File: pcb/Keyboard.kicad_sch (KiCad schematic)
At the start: 63 parts

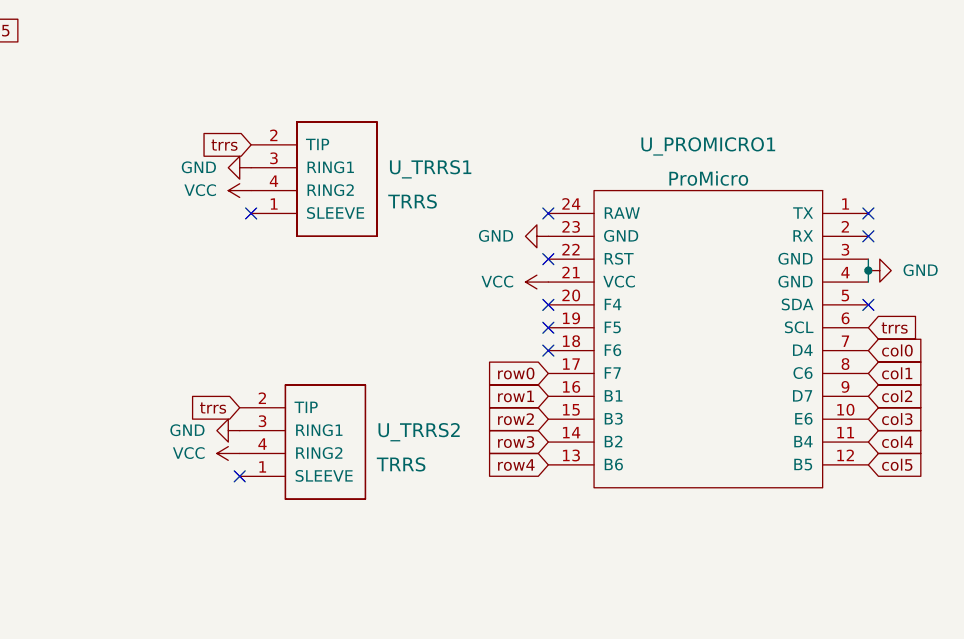
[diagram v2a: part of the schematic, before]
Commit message: wip
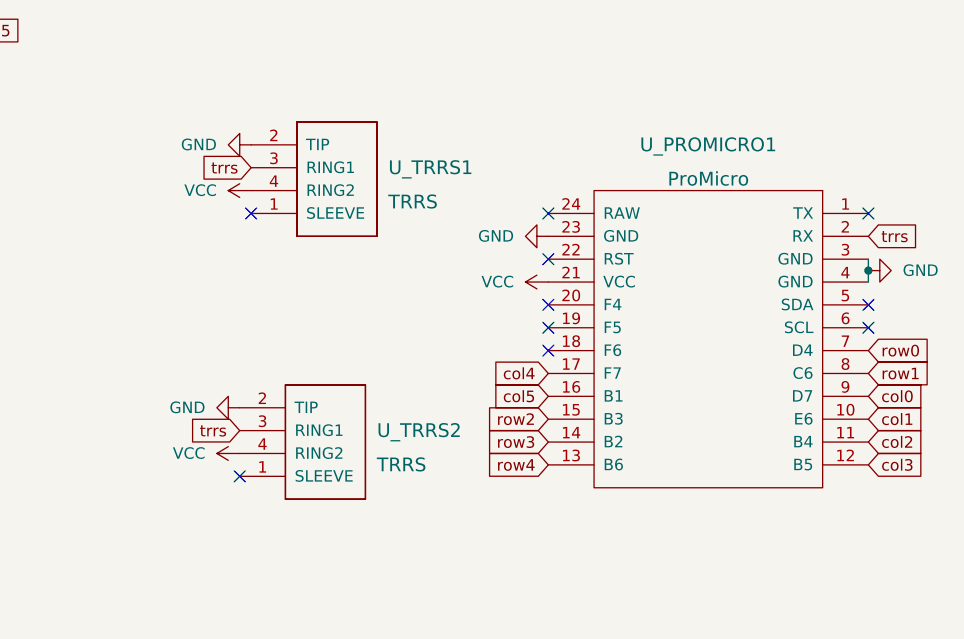
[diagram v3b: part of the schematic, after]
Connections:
- net GND: now also U_TRRS1.2 (TIP), U_TRRS2.2 (TIP); no longer U_TRRS1.3 (RING1), U_TRRS2.3 (RING1)
- net col0: now also U_PROMICRO1.9 (D7); no longer U_PROMICRO1.7 (D4)
- net col1: now also U_PROMICRO1.10 (E6); no longer U_PROMICRO1.8 (C6)
- net col2: now also U_PROMICRO1.11 (B4); no longer U_PROMICRO1.9 (D7)
- net col3: now also U_PROMICRO1.12 (B5); no longer U_PROMICRO1.10 (E6)
- net col4: now also U_PROMICRO1.17 (F7); no longer U_PROMICRO1.11 (B4)
- net col5: now also U_PROMICRO1.16 (B1); no longer U_PROMICRO1.12 (B5)
- net row0: now also U_PROMICRO1.7 (D4); no longer U_PROMICRO1.17 (F7)
- net row1: now also U_PROMICRO1.8 (C6); no longer U_PROMICRO1.16 (B1)
- net trrs: now also U_PROMICRO1.2 (RX), U_TRRS1.3 (RING1), U_TRRS2.3 (RING1); no longer U_PROMICRO1.6 (SCL), U_TRRS1.2 (TIP), U_TRRS2.2 (TIP)
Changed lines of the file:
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@@
   (no_connect (at 227.33 43.18))
   (no_connect (at 262.89 53.34))
-  (no_connect (at 262.89 45.72))
   (no_connect (at 262.89 43.18))
   (no_connect (at 227.33 58.42))
+  (no_connect (at 262.89 55.88))
   (no_connect (at 193.04 72.39))
   (no_connect (at 194.31 43.18))
@@
     (stroke (width 0) (type default) (color 0 0 0 0))
   )
-  (global_label "col5" (shape input) (at 262.89 71.12 0) (fields_autoplaced)
+  (global_label "col5" (shape input) (at 227.33 63.5 180) (fields_autoplaced)
+    (effects (font (size 1.27 1.27)) (justify right))
+    (property "Intersheet References" "${INTERSHEET_REFS}" (id 0) (at 220.8045 63.4206 0)
+      (effects (font (size 1.27 1.27)) (justify right) hide)
+    )
+  )
+  (global_label "col3" (shape input) (at 262.89 71.12 0) (fields_autoplaced)
     (effects (font (size 1.27 1.27)) (justify left))
     (property "Intersheet References" "${INTERSHEET_REFS}" (id 0) (at 269.4155 71.0406 0)
-      (effects (font (size 1.27 1.27)) (justify left) hide)
-    )
-  )
-  (global_label "col3" (shape input) (at 262.89 66.04 0) (fields_autoplaced)
-    (effects (font (size 1.27 1.27)) (justify left))
-    (property "Intersheet References" "${INTERSHEET_REFS}" (id 0) (at 269.4155 65.9606 0)
       (effects (font (size 1.27 1.27)) (justify left) hide)
     )
@@
     )
   )
-  (global_label "trrs" (shape input) (at 194.31 35.56 180) (fields_autoplaced)
+  (global_label "trrs" (shape input) (at 194.31 38.1 180) (fields_autoplaced)
     (effects (font (size 1.27 1.27)) (justify right))
-    (property "Intersheet References" "${INTERSHEET_REFS}" (id 0) (at 188.5707 35.4806 0)
+    (property "Intersheet References" "${INTERSHEET_REFS}" (id 0) (at 188.5707 38.0206 0)
       (effects (font (size 1.27 1.27)) (justify right) hide)
     )
@@
     )
   )
-  (global_label "trrs" (shape input) (at 262.89 55.88 0) (fields_autoplaced)
+  (global_label "trrs" (shape input) (at 262.89 45.72 0) (fields_autoplaced)
     (effects (font (size 1.27 1.27)) (justify left))
-    (property "Intersheet References" "${INTERSHEET_REFS}" (id 0) (at 268.6293 55.8006 0)
+    (property "Intersheet References" "${INTERSHEET_REFS}" (id 0) (at 268.6293 45.6406 0)
       (effects (font (size 1.27 1.27)) (justify left) hide)
     )
@@
     )
   )
-  (global_label "col2" (shape input) (at 262.89 63.5 0) (fields_autoplaced)
+  (global_label "col2" (shape input) (at 262.89 68.58 0) (fields_autoplaced)
     (effects (font (size 1.27 1.27)) (justify left))
-    (property "Intersheet References" "${INTERSHEET_REFS}" (id 0) (at 269.4155 63.4206 0)
+    (property "Intersheet References" "${INTERSHEET_REFS}" (id 0) (at 269.4155 68.5006 0)
       (effects (font (size 1.27 1.27)) (justify left) hide)
     )
@@
     )
   )
-  (global_label "col4" (shape input) (at 262.89 68.58 0) (fields_autoplaced)
-    (effects (font (size 1.27 1.27)) (justify left))
-    (property "Intersheet References" "${INTERSHEET_REFS}" (id 0) (at 269.4155 68.5006 0)
-      (effects (font (size 1.27 1.27)) (justify left) hide)
+  (global_label "col4" (shape input) (at 227.33 60.96 180) (fields_autoplaced)
+    (effects (font (size 1.27 1.27)) (justify right))
+    (property "Intersheet References" "${INTERSHEET_REFS}" (id 0) (at 220.8045 60.8806 0)
+      (effects (font (size 1.27 1.27)) (justify right) hide)
     )
   )
@@
     )
   )
-  (global_label "row0" (shape input) (at 227.33 60.96 180) (fields_autoplaced)
-    (effects (font (size 1.27 1.27)) (justify right))
-    (property "Intersheet References" "${INTERSHEET_REFS}" (id 0) (at 220.4417 60.8806 0)
-      (effects (font (size 1.27 1.27)) (justify right) hide)
+  (global_label "row0" (shape input) (at 262.89 58.42 0) (fields_autoplaced)
+    (effects (font (size 1.27 1.27)) (justify left))
+    (property "Intersheet References" "${INTERSHEET_REFS}" (id 0) (at 269.7783 58.3406 0)
+      (effects (font (size 1.27 1.27)) (justify left) hide)
     )
   )
@@
     )
   )
-  (global_label "col0" (shape input) (at 262.89 58.42 0) (fields_autoplaced)
+  (global_label "col0" (shape input) (at 262.89 63.5 0) (fields_autoplaced)
     (effects (font (size 1.27 1.27)) (justify left))
-    (property "Intersheet References" "${INTERSHEET_REFS}" (id 0) (at 269.4155 58.3406 0)
+    (property "Intersheet References" "${INTERSHEET_REFS}" (id 0) (at 269.4155 63.4206 0)
       (effects (font (size 1.27 1.27)) (justify left) hide)
     )
   )
-  (global_label "trrs" (shape input) (at 193.04 64.77 180) (fields_autoplaced)
+  (global_label "trrs" (shape input) (at 193.04 67.31 180) (fields_autoplaced)
     (effects (font (size 1.27 1.27)) (justify right))
-    (property "Intersheet References" "${INTERSHEET_REFS}" (id 0) (at 187.3007 64.6906 0)
+    (property "Intersheet References" "${INTERSHEET_REFS}" (id 0) (at 187.3007 67.2306 0)
       (effects (font (size 1.27 1.27)) (justify right) hide)
     )
   )
-  (global_label "row1" (shape input) (at 227.33 63.5 180) (fields_autoplaced)
-    (effects (font (size 1.27 1.27)) (justify right))
-    (property "Intersheet References" "${INTERSHEET_REFS}" (id 0) (at 220.4417 63.4206 0)
-      (effects (font (size 1.27 1.27)) (justify right) hide)
+  (global_label "row1" (shape input) (at 262.89 60.96 0) (fields_autoplaced)
+    (effects (font (size 1.27 1.27)) (justify left))
+    (property "Intersheet References" "${INTERSHEET_REFS}" (id 0) (at 269.7783 60.8806 0)
+      (effects (font (size 1.27 1.27)) (justify left) hide)
     )
   )
@@
     )
   )
-  (global_label "col1" (shape input) (at 262.89 60.96 0) (fields_autoplaced)
+  (global_label "col1" (shape input) (at 262.89 66.04 0) (fields_autoplaced)
     (effects (font (size 1.27 1.27)) (justify left))
-    (property "Intersheet References" "${INTERSHEET_REFS}" (id 0) (at 269.4155 60.8806 0)
+    (property "Intersheet References" "${INTERSHEET_REFS}" (id 0) (at 269.4155 65.9606 0)
       (effects (font (size 1.27 1.27)) (justify left) hide)
     )
@@
     (pin "1")
   )
-  (symbol (lib_id "power:GND") (at 193.04 67.31 270) (unit 1)
-    (in_bom yes) (on_board yes) (fields_autoplaced)
-    (property "Reference" "#PWR0102" (id 0) (at 186.69 67.31 0)
-      (effects (font (size 1.27 1.27)) hide)
-    )
-    (property "Value" "GND" (id 1) (at 189.23 67.3099 90)
-      (effects (font (size 1.27 1.27)) (justify right))
-    )
-    (property "Footprint" "" (id 2) (at 193.04 67.31 0)
-      (effects (font (size 1.27 1.27)) hide)
-    )
-    (property "Datasheet" "" (id 3) (at 193.04 67.31 0)
+  (symbol (lib_id "power:GND") (at 193.04 64.77 270) (unit 1)
+    (in_bom yes) (on_board yes)
+    (property "Reference" "#PWR0102" (id 0) (at 186.69 64.77 0)
+      (effects (font (size 1.27 1.27)) hide)
+    )
+    (property "Value" "GND" (id 1) (at 189.23 64.7699 90)
+      (effects (font (size 1.27 1.27)) (justify right))
+    )
+    (property "Footprint" "" (id 2) (at 193.04 64.77 0)
+      (effects (font (size 1.27 1.27)) hide)
+    )
+    (property "Datasheet" "" (id 3) (at 193.04 64.77 0)
       (effects (font (size 1.27 1.27)) hide)
     )
@@
     (pin "2")
   )
-  (symbol (lib_id "power:GND") (at 194.31 38.1 270) (unit 1)
-    (in_bom yes) (on_board yes) (fields_autoplaced)
-    (property "Reference" "#PWR0104" (id 0) (at 187.96 38.1 0)
-      (effects (font (size 1.27 1.27)) hide)
-    )
-    (property "Value" "GND" (id 1) (at 190.5 38.0999 90)
-      (effects (font (size 1.27 1.27)) (justify right))
-    )
-    (property "Footprint" "" (id 2) (at 194.31 38.1 0)
-      (effects (font (size 1.27 1.27)) hide)
-    )
-    (property "Datasheet" "" (id 3) (at 194.31 38.1 0)
-      (effects (font (size 1.27 1.27)) hide)
-    )
+  (symbol (lib_id "power:GND") (at 194.31 35.56 270) (unit 1)
+    (in_bom yes) (on_board yes) (fields_autoplaced)
+    (property "Reference" "#PWR0104" (id 0) (at 187.96 35.56 0)
+      (effects (font (size 1.27 1.27)) hide)
+    )
+    (property "Value" "GND" (id 1) (at 190.5 35.5599 90)
+      (effects (font (size 1.27 1.27)) (justify right))
+    )
+    (property "Footprint" "" (id 2) (at 194.31 35.56 0)
+      (effects (font (size 1.27 1.27)) hide)
+    )
+    (property "Datasheet" "" (id 3) (at 194.31 35.56 0)
+      (effects (font (size 1.27 1.27)) hide)
+    )

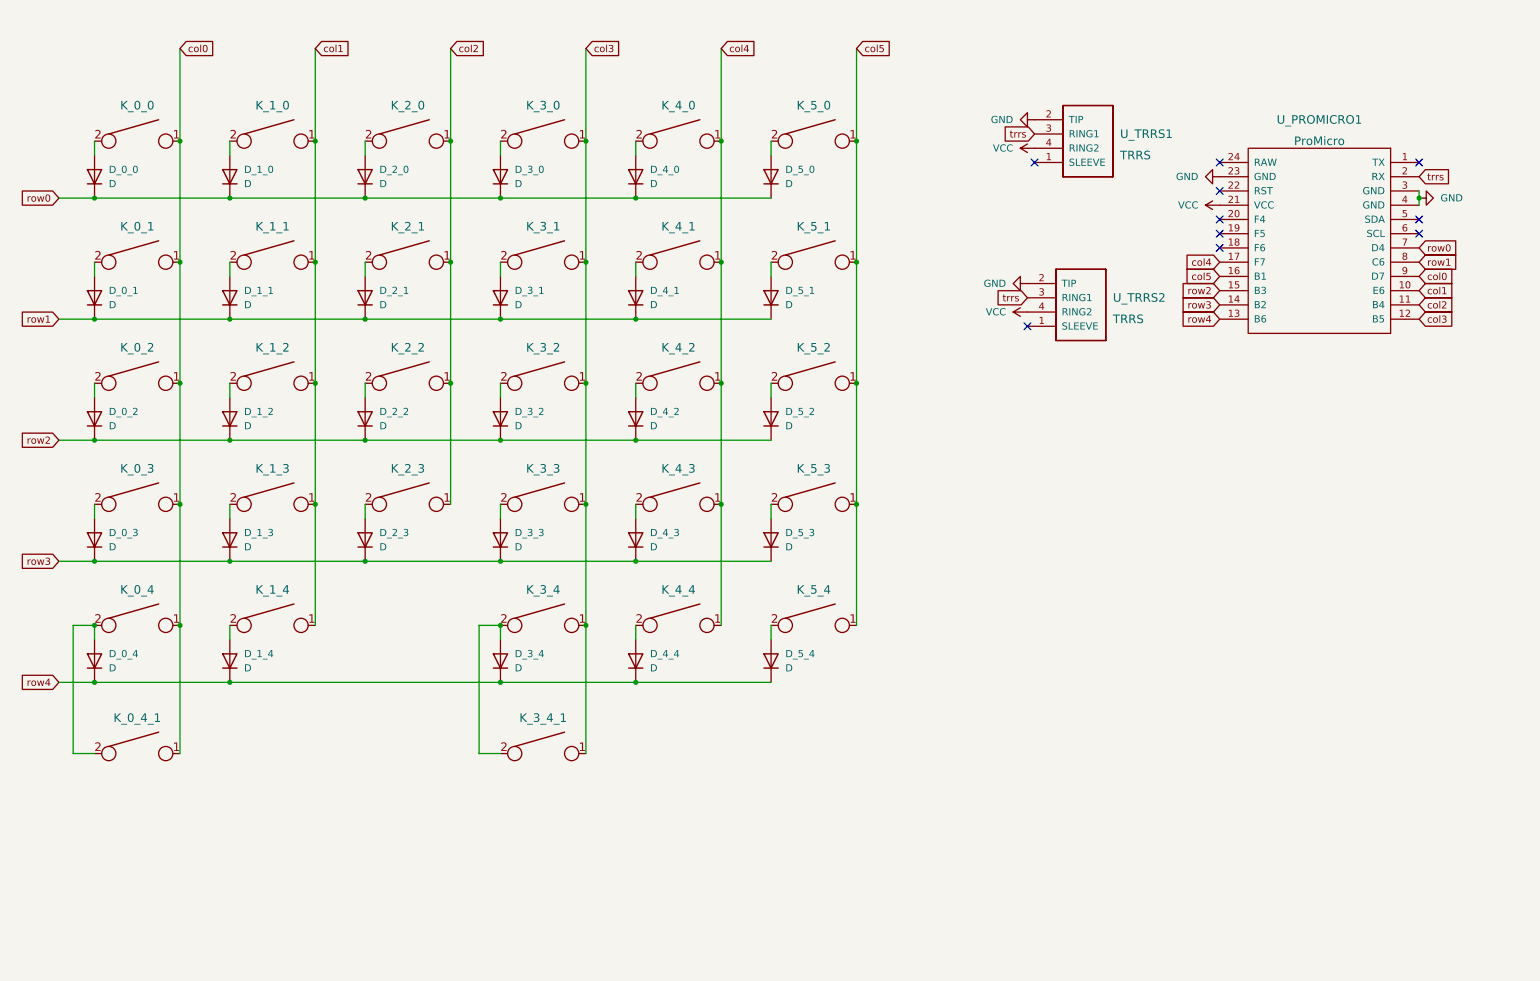
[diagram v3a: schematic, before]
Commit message: wip
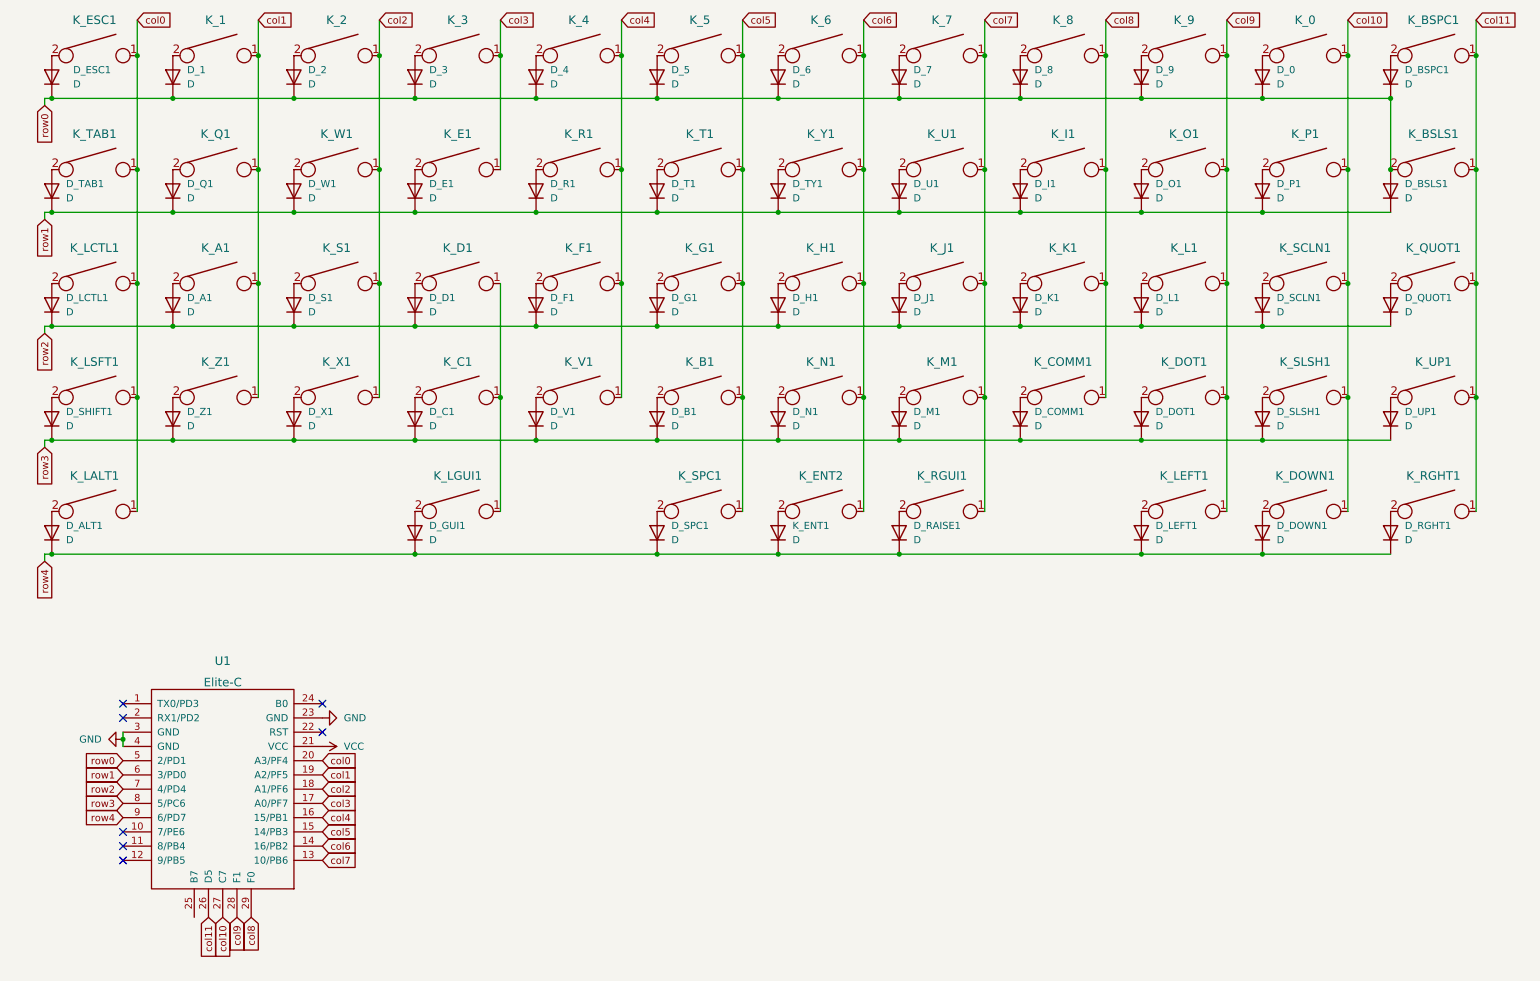
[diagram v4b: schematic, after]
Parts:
- removed D_0_4, D_1_4, D_3_4, D_4_4, D_5_4: D, keyboard_parts:D_SOD123, symbol Device:D
- removed K_0_4, K_0_4_1, K_1_4, K_3_4, K_3_4_1, K_4_4, K_5_4: KEYSW, Switch_Keyboard_Hotswap_Kailh:SW_Hotswap_Kailh_Choc_V1_1.00u, symbol keyboard_parts:KEYSW
- removed U_PROMICRO1: ProMicro, promicro:ProMicro, symbol promicro:ProMicro
- removed U_TRRS1, U_TRRS2: TRRS, Keebio-Parts:TRRS-PJ-320A, symbol keebio:TRRS
- added D_0, D_6, D_7, D_8, D_9, D_ALT1, D_BSLS1, D_BSPC1, D_COMM1, D_DOT1, D_DOWN1, D_GUI1, D_H1, D_I1, D_J1, D_K1, D_L1, D_LEFT1, D_M1, D_N1, D_O1, D_P1, D_QUOT1, D_RAISE1, D_RGHT1, D_SCLN1, D_SLSH1, D_SPC1, D_TY1, D_U1, D_UP1, K_ENT1: D, keyboard_parts:D_SOD123, symbol Device:D
- added K_0, K_6, K_7, K_8, K_9, K_BSLS1, K_BSPC1, K_COMM1, K_DOT1, K_DOWN1, K_ENT2, K_H1, K_I1, K_J1, K_K1, K_L1, K_LALT1, K_LEFT1, K_LGUI1, K_M1, K_N1, K_O1, K_P1, K_QUOT1, K_RGHT1, K_RGUI1, K_SCLN1, K_SLSH1, K_SPC1, K_U1, K_UP1, K_Y1: KEYSW, Switch_Keyboard_Hotswap_Kailh:SW_Hotswap_Kailh_Choc_V1_1.00u, symbol keyboard_parts:KEYSW
- added U1: Elite-C, Keebio-Parts:Elite-C, symbol keebio:Elite-C
- renumbered D_1_0 to D_1, D_2_0 to D_2, D_3_0 to D_3, D_4_0 to D_4, D_5_0 to D_5, D_1_2 to D_A1, D_5_3 to D_B1, D_3_3 to D_C1, D_3_2 to D_D1, D_3_1 to D_E1, D_0_0 to D_ESC1, D_4_2 to D_F1, D_5_2 to D_G1, D_0_2 to D_LCTL1, D_1_1 to D_Q1, D_4_1 to D_R1, D_2_2 to D_S1, D_0_3 to D_SHIFT1, D_5_1 to D_T1, D_0_1 to D_TAB1, D_4_3 to D_V1, D_2_1 to D_W1, D_2_3 to D_X1, D_1_3 to D_Z1, K_1_0 to K_1, K_2_0 to K_2, K_3_0 to K_3, K_4_0 to K_4, K_5_0 to K_5, K_1_2 to K_A1, K_5_3 to K_B1, K_3_3 to K_C1, K_3_2 to K_D1, K_3_1 to K_E1, K_0_0 to K_ESC1, K_4_2 to K_F1, K_5_2 to K_G1, K_0_2 to K_LCTL1, K_0_3 to K_LSFT1, K_1_1 to K_Q1, K_4_1 to K_R1, K_2_2 to K_S1, K_5_1 to K_T1, K_0_1 to K_TAB1, K_4_3 to K_V1, K_2_1 to K_W1, K_2_3 to K_X1, K_1_3 to K_Z1
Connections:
- net GND: now also U1.23 (GND), U1.3 (GND), U1.4 (GND)
- net VCC: now also U1.21 (VCC)
- net col0: now also K_LALT1.1, U1.20 (A3/PF4)
- net col1: now also U1.19 (A2/PF5)
- net col2: now also U1.18 (A1/PF6)
- net col3: now also U1.17 (A0/PF7); no longer K_C1.1, K_D1.1
- net col4: now also U1.16 (15/PB1)
- net col5: now also K_SPC1.1, U1.15 (14/PB3)
- net row0: now also D_0.1 (K), D_6.1 (K), D_7.1 (K), D_8.1 (K), D_9.1 (K), D_BSLS1.2 (A), D_BSPC1.1 (K), K_BSLS1.2, U1.5 (2/PD1)
- net row1: now also D_BSLS1.1 (K), D_I1.1 (K), D_O1.1 (K), D_P1.1 (K), D_TY1.1 (K), D_U1.1 (K), U1.6 (3/PD0)
- net row2: now also D_H1.1 (K), D_J1.1 (K), D_K1.1 (K), D_L1.1 (K), D_QUOT1.1 (K), D_SCLN1.1 (K), U1.7 (4/PD4)
- net row3: now also D_COMM1.1 (K), D_DOT1.1 (K), D_M1.1 (K), D_N1.1 (K), D_SLSH1.1 (K), D_UP1.1 (K), U1.8 (5/PC6)
- net row4: now also D_ALT1.1 (K), D_DOWN1.1 (K), D_GUI1.1 (K), D_LEFT1.1 (K), D_RAISE1.1 (K), D_RGHT1.1 (K), D_SPC1.1 (K), K_ENT1.1 (K), U1.9 (6/PD7)
- new net: D_6.2 (A), K_6.2
- new net: D_ALT1.2 (A), K_LALT1.2
- new net: D_SPC1.2 (A), K_SPC1.2
- new net: D_U1.2 (A), K_U1.2
- new net: D_QUOT1.2 (A), K_QUOT1.2
- new net: D_LEFT1.2 (A), K_LEFT1.2
- new net: D_SLSH1.2 (A), K_SLSH1.2
- new net: D_O1.2 (A), K_O1.2
- new net: D_SCLN1.2 (A), K_SCLN1.2
- new net: D_TY1.2 (A), K_Y1.2
- new net: D_DOWN1.2 (A), K_DOWN1.2
- new net: D_H1.2 (A), K_H1.2
- new net: D_BSPC1.2 (A), K_BSPC1.2
- new net: D_M1.2 (A), K_M1.2
- new net: D_7.2 (A), K_7.2
- new net: D_8.2 (A), K_8.2
- new net: D_P1.2 (A), K_P1.2
- new net: D_UP1.2 (A), K_UP1.2
- new net: D_K1.2 (A), K_K1.2
- new net: K_C1.1, K_D1.1, K_LGUI1.1
- new net: D_RGHT1.2 (A), K_RGHT1.2
- new net: D_GUI1.2 (A), K_LGUI1.2
- new net: D_J1.2 (A), K_J1.2
- new net: D_I1.2 (A), K_I1.2
- new net: D_L1.2 (A), K_L1.2
- new net: D_RAISE1.2 (A), K_RGUI1.2
- new net: D_DOT1.2 (A), K_DOT1.2
- new net: D_COMM1.2 (A), K_COMM1.2
- new net: D_0.2 (A), K_0.2
- new net: D_9.2 (A), K_9.2
- new net: K_ENT1.2 (A), K_ENT2.2
- new net: D_N1.2 (A), K_N1.2
- new net col10: K_0.1, K_DOWN1.1, K_P1.1, K_SCLN1.1, K_SLSH1.1, U1.27 (C7)
- new net col11: K_BSLS1.1, K_BSPC1.1, K_QUOT1.1, K_RGHT1.1, K_UP1.1, U1.26 (D5)
- new net col6: K_6.1, K_ENT2.1, K_H1.1, K_N1.1, K_Y1.1, U1.14 (16/PB2)
- new net col7: K_7.1, K_J1.1, K_M1.1, K_RGUI1.1, K_U1.1, U1.13 (10/PB6)
- new net col8: K_8.1, K_COMM1.1, K_I1.1, K_K1.1, U1.29 (F0)
- new net col9: K_9.1, K_DOT1.1, K_L1.1, K_LEFT1.1, K_O1.1, U1.28 (F1)
- no-connect marks 10 -> 7
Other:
- moved on the sheet: D_1, D_2, D_3, D_4, D_5, D_A1, D_B1, D_C1, D_D1, D_E1, D_ESC1, D_F1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
